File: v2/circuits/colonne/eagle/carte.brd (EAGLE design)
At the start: 105.4 x 45.4 mm, 15 parts, among them Q1 TIP31C, Q2 TIP31C, Q3 TIP31C, Q4 TIP30, Q5 TIP30, Q6 TIP30, X1 MKS1854-6-0-404, X2 MKS1854-6-0-404, X3 MKS1854-6-0-404

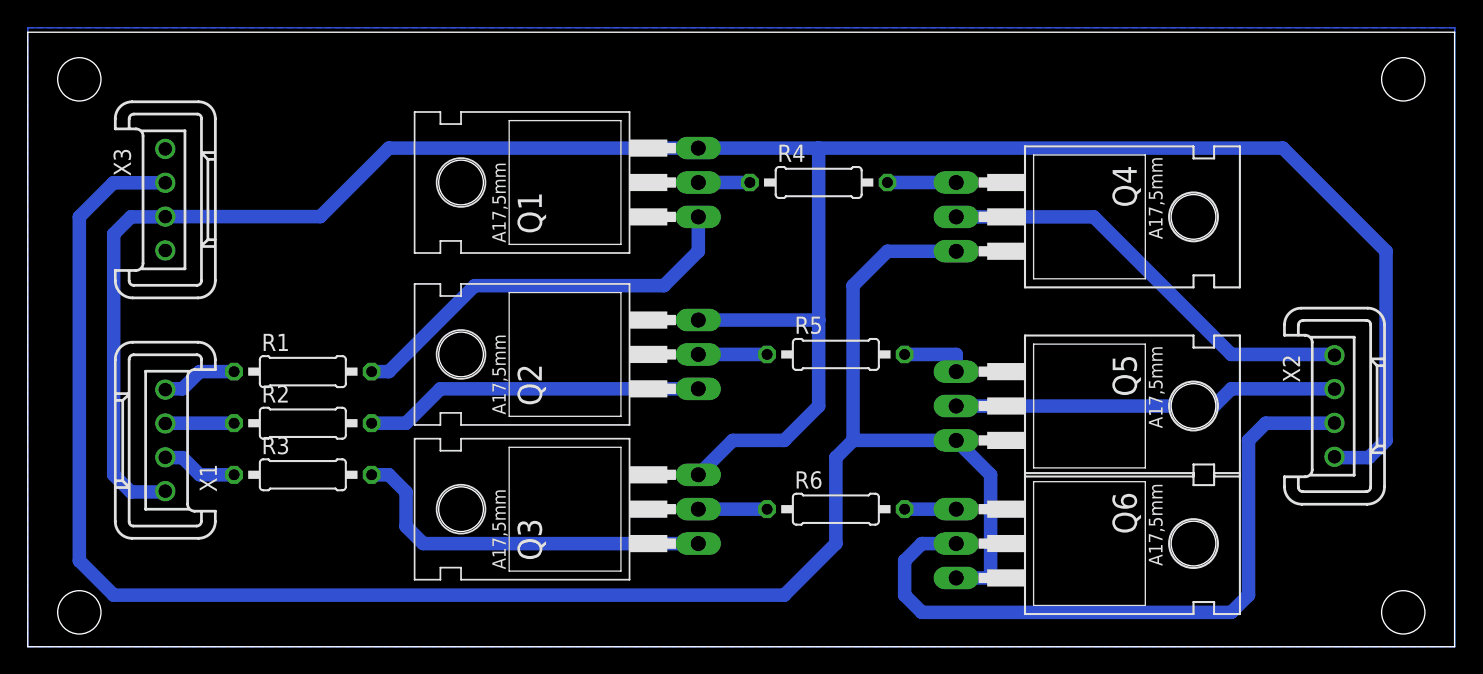
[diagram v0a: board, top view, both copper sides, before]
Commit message: added boards
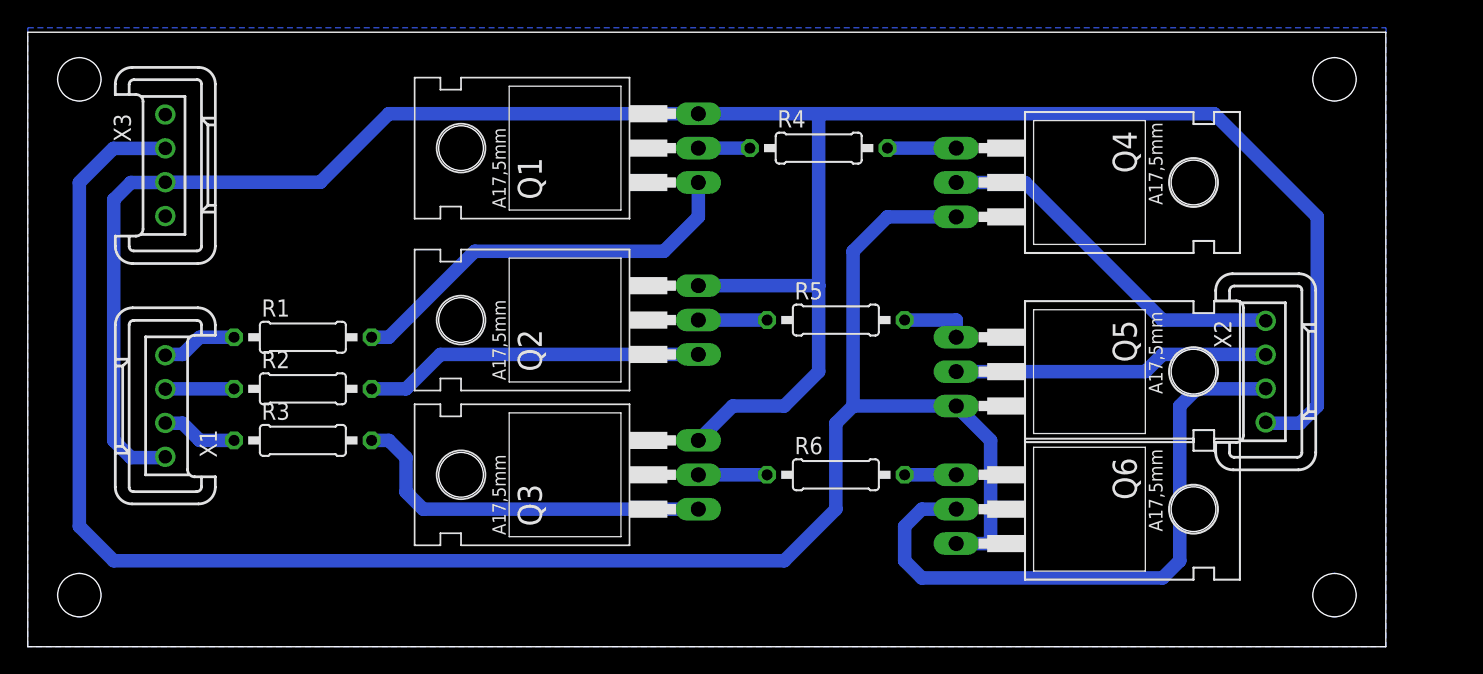
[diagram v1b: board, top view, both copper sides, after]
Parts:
- moved X2 5.68 mm to (88.9, 54.6)
- moved Q1 2.54 mm to (40.6, 71.1)
- moved Q6 2.54 mm to (72.4, 44.5)
- moved R2 2.54 mm to (17.8, 53.3)
- moved R4 2.54 mm to (55.9, 71.1)
- moved Q2 2.54 mm to (40.6, 58.4)
- moved Q3 2.54 mm to (40.6, 47.0)
- moved Q5 2.54 mm to (72.4, 54.6)
- moved R1 2.54 mm to (17.8, 57.1)
- moved R3 2.54 mm to (17.8, 49.5)
- moved R5 2.54 mm to (57.1, 58.4)
- moved R6 2.54 mm to (57.1, 47.0)
- moved X1 2.54 mm to (7.62, 52.1)
- moved Q4 2.54 mm to (72.4, 68.6)
- moved X3 2.54 mm to (7.62, 69.8)
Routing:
- net N$11: track 302.3 -> 0.00 mm
- net N$10: track 179.3 -> 174.2 mm
- net N$31: track 0.00 -> 5.08 mm
- net N$16: track 32.2 -> 27.1 mm
- net N$28: track 0.00 -> 5.08 mm
- net N$30: track 0.00 -> 5.08 mm
- net N$17: track 28.5 -> 23.4 mm
- net N$29: track 0.00 -> 5.08 mm
- net N$18: track 51.6 -> 46.6 mm
- net N$22: track 2.54 -> 0.00 mm
- net N$20: track 2.54 -> 0.00 mm
- net N$23: track 2.54 -> 0.00 mm
- net N$21: track 2.54 -> 0.00 mm
- net N$26: track 2.54 -> 0.00 mm
- net N$25: track 2.54 -> 0.00 mm
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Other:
- board size 105.4 x 45.4 mm -> 100.3 x 45.4 mm
